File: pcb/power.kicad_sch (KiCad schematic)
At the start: 7 parts, among them U4 TPS61023DRLR

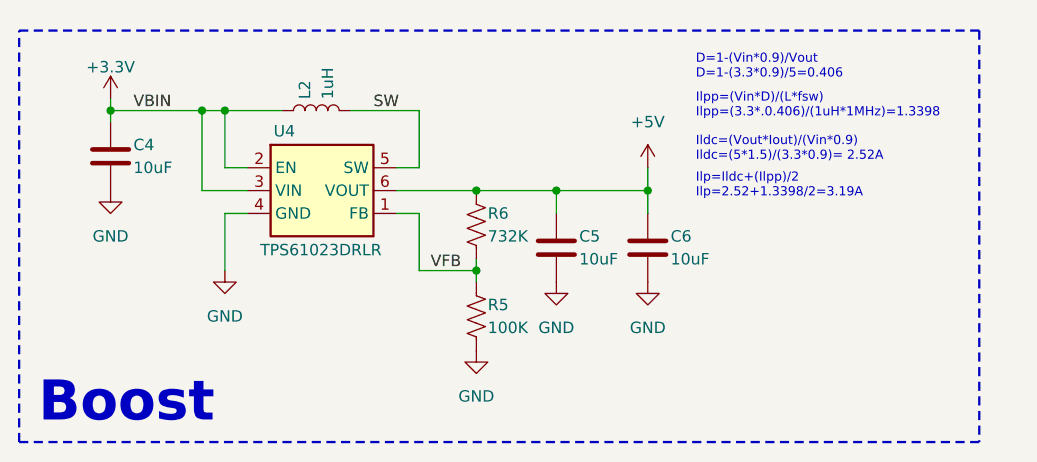
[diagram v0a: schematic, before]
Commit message: initial checkin
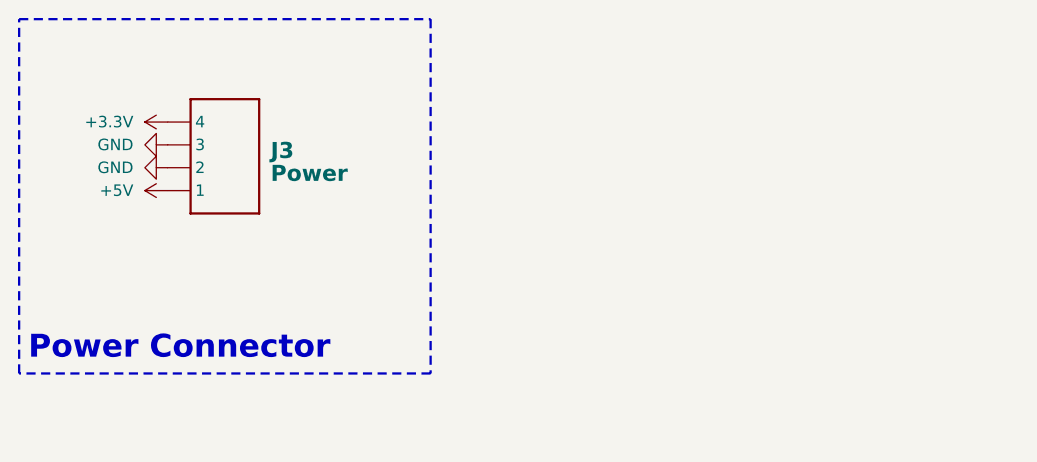
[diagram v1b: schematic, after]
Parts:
- removed C4, C5, C6: 10uF, Capacitor_SMD:C_0603_1608Metric, symbol Device:C
- removed L2: 1uH, Inductor_SMD:L_Wuerth_MAPI-2010, symbol Device:L
- removed R5: 100K, Resistor_SMD:R_0603_1608Metric, symbol Device:R_US
- removed R6: 732K, Resistor_SMD:R_0603_1608Metric, symbol Device:R_US
- removed U4: TPS61023DRLR, CRGM Power:SOTFL50P160X60-6N, symbol CRGM Power:TPS61023DRLR
- added J3: Power, Connector_JST:JST_SH_SM04B-SRSS-TB_1x04-1MP_P1.00mm_Horizontal, symbol CRGM Connector:JST-SH-4
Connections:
- net +3.3V: now also J3.4
- net +5V: now also J3.1
- net GND: now also J3.2, J3.3
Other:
- note added: "Power Connector"
- note removed: "Boost"
- note removed: "D=1-(Vin*0.9)/Vout D=1-(3.3*0.9)/5=0.406"
- note removed: "Ildc=(Vout*Iout)/(Vin*0.9) Ildc=(5*1.5)/(3.3*0.9)= 2.52A"
- note removed: "Ilp=Ildc+(Ilpp)/2 Ilp=2.52+1.3398/2=3.19A"
- note removed: "Ilpp=(Vin*D)/(L*fsw) Ilpp=(3.3*.0.406)/(1uH*1MHz)=1.3398"
